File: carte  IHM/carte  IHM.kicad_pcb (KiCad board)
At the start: 2 copper layers, 36.4 x 26.4 mm, 12 parts, among them J1 tirette, J2 UART CP, J3 init, J4 Conn_01x02, U1 XIAO-ESP32-S3-DIP, U2 TFT_320x240

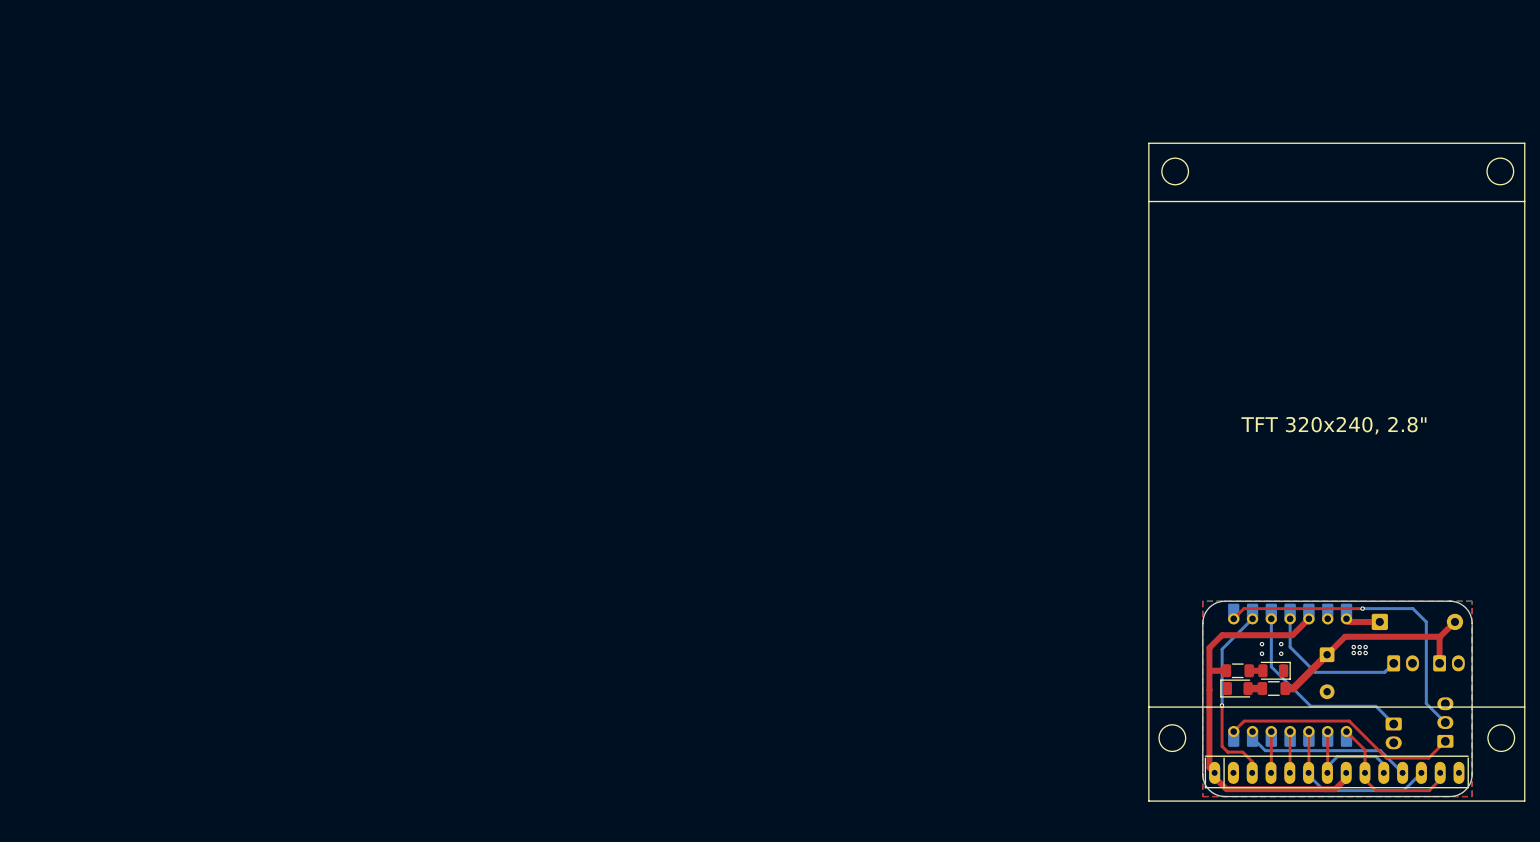
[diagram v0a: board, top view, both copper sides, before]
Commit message: v2
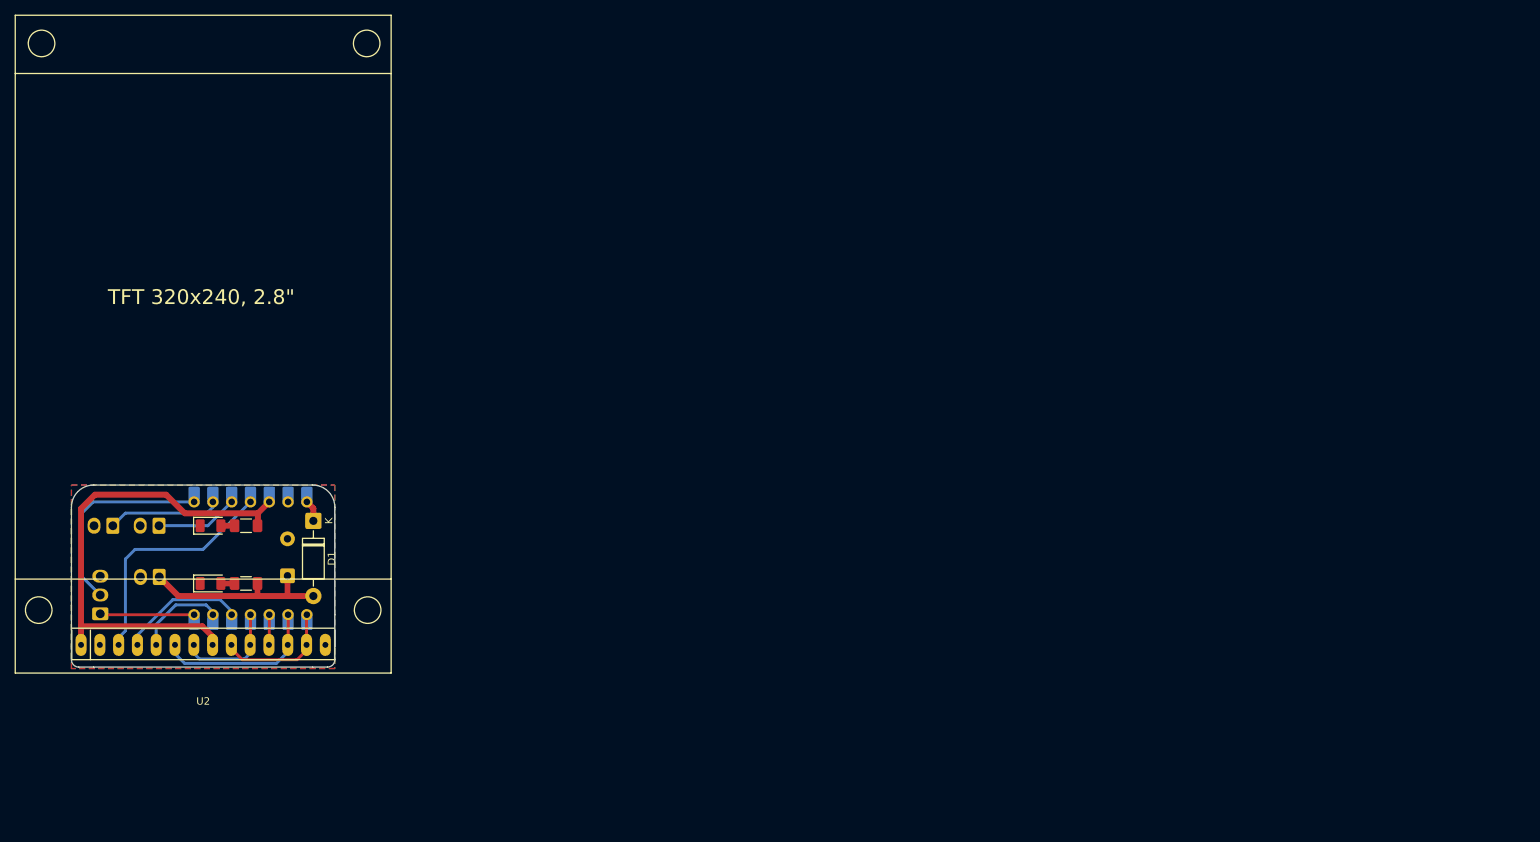
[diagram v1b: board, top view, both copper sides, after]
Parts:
- D1: moved to F.Cu
- moved J2 182.6 mm to (26.2, 95.3)
- moved J3 175.2 mm to (27.9, 83.4), turned to 180 degrees
- moved J4 173.4 mm to (34.2, 90.3), turned to 180 degrees
- moved J1 167.9 mm to (34.1, 83.4), turned to 180 degrees
- moved U2 154.2 mm to (40.1, 99.5)
- moved D3 145.0 mm to (41.1, 83.4), turned to 0 degrees
- moved D1 144.8 mm to (55.0, 82.7), turned to -90 degrees
- moved U1 141.4 mm to (46.5, 87.8)
- moved C5 140.9 mm to (51.5, 90.2), turned to 90 degrees
- moved R5 139.6 mm to (45.9, 91.2)
- moved D2 139.5 mm to (41.1, 91.2)
- moved R3 135.5 mm to (45.9, 83.4), turned to 180 degrees
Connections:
- U1 pad 10: init -> TIRETTE
- U1 pad 11: TIRETTE -> CS (écran)
- U1 pad 2: SCK -> MOSI
- U1 pad 3: MOSI -> CS (touch)
- U1 pad 4: DC -> SCK
- U1 pad 6: CS (touch) -> DC
- U1 pad 9: CS (écran) -> init
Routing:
- net RX: track 32.2 -> 12.7 mm
- net CS (touch): track 22.2 -> 4.10 mm
- net TX: track 42.0 -> 27.9 mm, vias 1 -> 0
- net +3.3V: track 54.8 -> 67.8 mm
- net RST: track 5.60 -> 17.1 mm
- net init: track 26.2 -> 15.3 mm
- net TIRETTE: track 19.7 -> 11.2 mm
- net DC: track 5.60 -> 12.3 mm
- net CS (écran): track 25.4 -> 32.1 mm, vias 1 -> 0
- net +5V: track 30.3 -> 26.3 mm
- net MISO: track 19.8 -> 16.6 mm
- net Net-(D1-K): track 4.67 -> 2.92 mm
- net SCK: track 16.2 -> 14.6 mm
- net GND: vias 10 -> 0
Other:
- board size 36.4 x 26.4 mm -> 35.6 x 24.6 mm

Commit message: fix
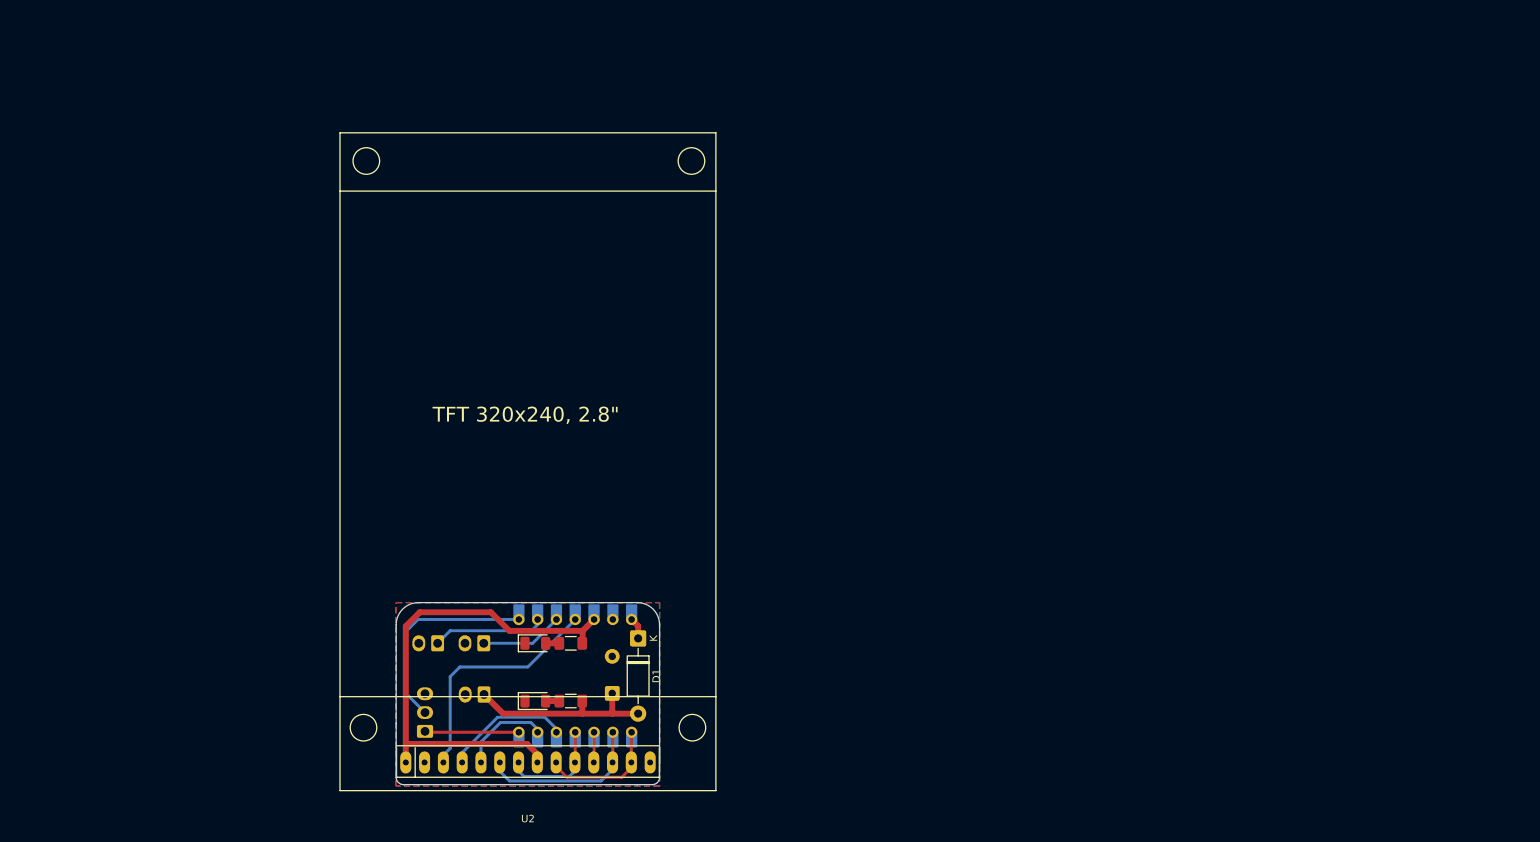
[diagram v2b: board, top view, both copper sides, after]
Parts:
- moved C5 46.7 mm to (95.4, 106.1)
- moved D1 46.7 mm to (98.9, 98.6)
- moved J1 46.7 mm to (78.0, 99.3)
- moved J2 46.7 mm to (70.1, 111.2)
- moved J3 46.7 mm to (71.8, 99.3)
- moved J4 46.7 mm to (78.1, 106.2)
- moved R3 46.7 mm to (89.8, 99.3)
- moved R5 46.7 mm to (89.8, 107.1)
- moved U1 46.7 mm to (90.4, 103.7)
- moved U2 46.7 mm to (84.0, 115.4)
- moved D2 46.7 mm to (85.0, 107.1)
- moved D3 46.7 mm to (85.0, 99.3)

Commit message: V1.1 avec étiquetage
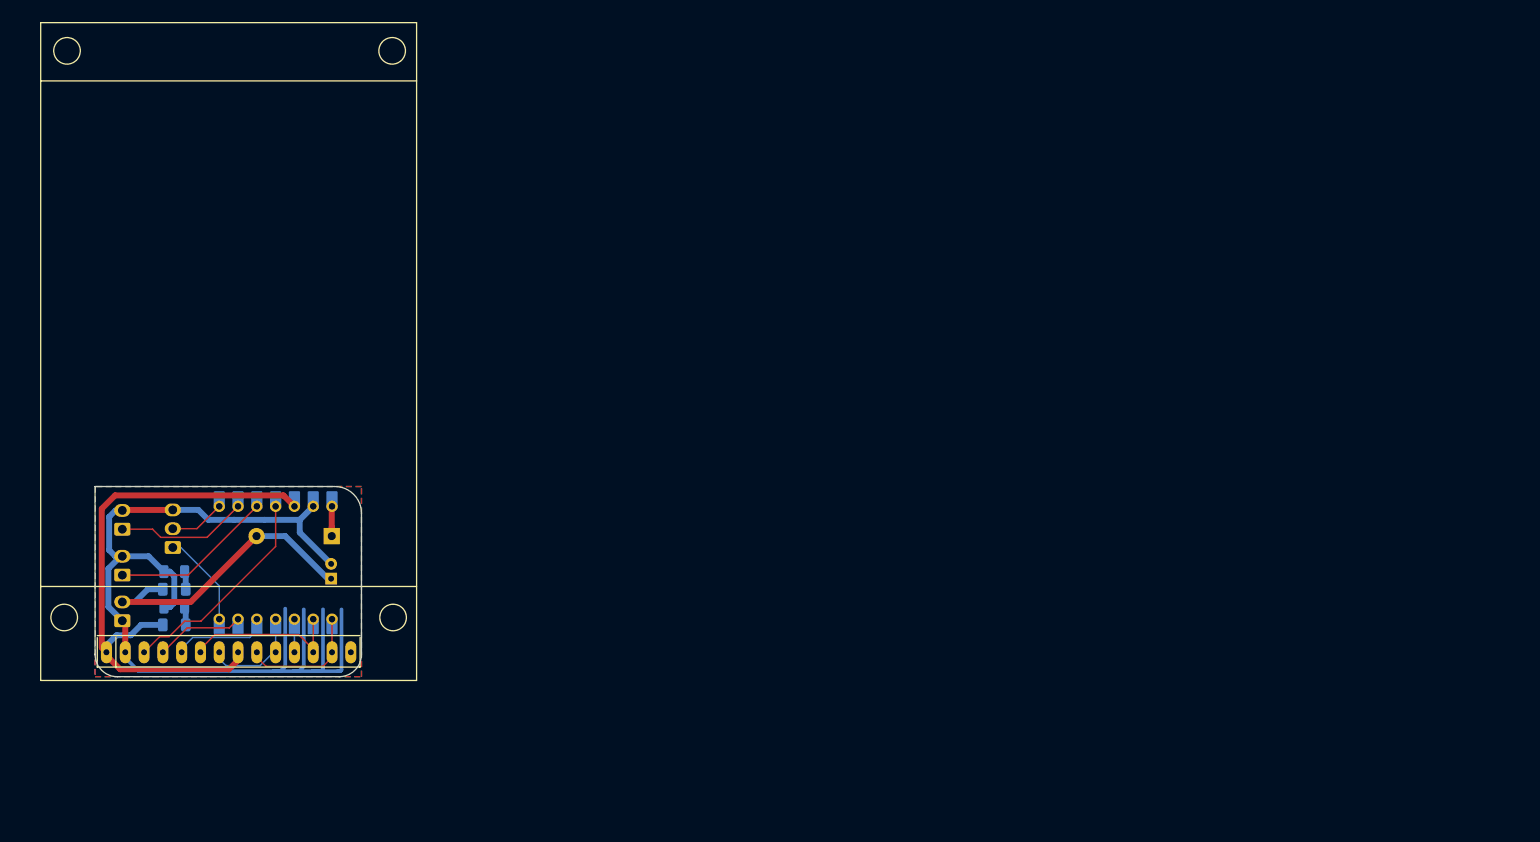
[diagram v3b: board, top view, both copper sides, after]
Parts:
- added G***: LOGO, LOGO, B.Cu at (41.8, 88.4)
- added kibuzzard-690E924D: G***, kibuzzard-690E924D, B.Cu at (32.6, 83.8)
- added kibuzzard-690E9271: G***, kibuzzard-690E9271, B.Cu at (25.8, 94.9)
- added kibuzzard-690E93A6: G***, kibuzzard-690E93A6, B.Cu at (36.2, 93.6)
- added kibuzzard-690E93B3: G***, kibuzzard-690E93B3, B.Cu at (36.2, 88.8)
- added kibuzzard-690E9406: G***, kibuzzard-690E9406, B.Cu at (36.2, 96.2)
- added kibuzzard-690E9406: G***, kibuzzard-690E9406, B.Cu at (36.2, 91.5)
- added kibuzzard-690E943A: G***, kibuzzard-690E943A, B.Cu at (36.2, 97.3)
- added kibuzzard-690E943A: G***, kibuzzard-690E943A, B.Cu at (36.2, 92.5)
- added kibuzzard-6910807D: G***, kibuzzard-6910807D, B.Cu at (44.8, 82.4)
- added kibuzzard-6910808E: G***, kibuzzard-6910808E, B.Cu at (44.8, 94.5)
- added kibuzzard-691080A1: G***, kibuzzard-691080A1, B.Cu at (42.3, 94.7)
- added kibuzzard-691080B6: G***, kibuzzard-691080B6, B.Cu at (47.4, 94.7)
- added kibuzzard-691080CB: G***, kibuzzard-691080CB, B.Cu at (49.9, 94.5)
- added kibuzzard-691080DD: G***, kibuzzard-691080DD, B.Cu at (52.4, 93.3)
- added kibuzzard-691080F8: G***, kibuzzard-691080F8, B.Cu at (55.0, 94.3)
- added kibuzzard-69108106: G***, kibuzzard-69108106, B.Cu at (57.5, 94.3)
- added kibuzzard-69108124: G***, kibuzzard-69108124, B.Cu at (47.4, 82.3)
- added kibuzzard-69108131: G***, kibuzzard-69108131, B.Cu at (42.3, 82.1)
- added kibuzzard-69108151: G***, kibuzzard-69108151, B.Cu at (49.9, 83.5)
- added kibuzzard-69108163: G***, kibuzzard-69108163, B.Cu at (52.4, 82.7)
- added kibuzzard-691084CF: G***, kibuzzard-691084CF, B.Cu at (25.8, 88.8)
- added kibuzzard-691084E9: G***, kibuzzard-691084E9, B.Cu at (25.8, 82.6)
- C5: footprint Capacitor_THT:CP_Radial_D10.0mm_P5.00mm -> Capacitor_THT:CP_Radial_D5.0mm_P2.00mm
- D1, D2, D3, R3, R5: moved to B.Cu
- moved R5 55.7 mm to (36.2, 92.0), turned to 0 degrees
- moved R3 53.6 mm to (36.2, 96.8), turned to 0 degrees
- moved D2 51.8 mm to (36.2, 89.6)
- moved J4 49.9 mm to (29.2, 96.2), turned to 90 degrees
- moved J1 49.7 mm to (29.2, 90.1), turned to 90 degrees
- moved D3 49.0 mm to (36.2, 94.4)
- moved J3 45.3 mm to (29.2, 83.9), turned to 90 degrees
- moved D1 43.7 mm to (57.5, 84.8), turned to 180 degrees
- moved U1 43.3 mm to (49.9, 88.4)
- moved U2 43.1 mm to (43.5, 100.5)
- moved J2 42.2 mm to (36.0, 86.3)
- moved C5 41.0 mm to (57.4, 90.6)
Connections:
- J4 pad 1: +5V -> GND
- J4 pad 2: GND -> +5V
- U1 pad 5: RST -> DC
- U1 pad 6: DC -> RST
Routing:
- net GND: track 0.00 -> 139.4 mm
- net TX: track 27.9 -> 7.53 mm
- net +5V: track 26.3 -> 40.5 mm
- net TIRETTE: track 11.2 -> 22.0 mm
- net +3.3V: track 67.8 -> 77.3 mm
- net RST: track 17.1 -> 12.0 mm
- net CS (écran): track 32.1 -> 29.1 mm
- net init: track 15.3 -> 17.8 mm
- net Net-(D1-K): track 2.92 -> 5.24 mm
- net Net-(D3-A): track 1.85 -> 2.46 mm
- net Net-(D2-A): track 1.85 -> 2.45 mm
- net MOSI: track 22.8 -> 22.2 mm
- net SCK: track 14.6 -> 14.1 mm
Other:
- board size 35.6 x 24.6 mm -> 36 x 25.7 mm
- board text added: "By Oscar Yosh GRIVELET"
- board text added: "Carte_IHM 2026_V1"
